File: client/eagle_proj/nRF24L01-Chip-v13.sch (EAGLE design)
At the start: 14 parts, among them IC1 7805DT, U2 ATMEGA328P-MU

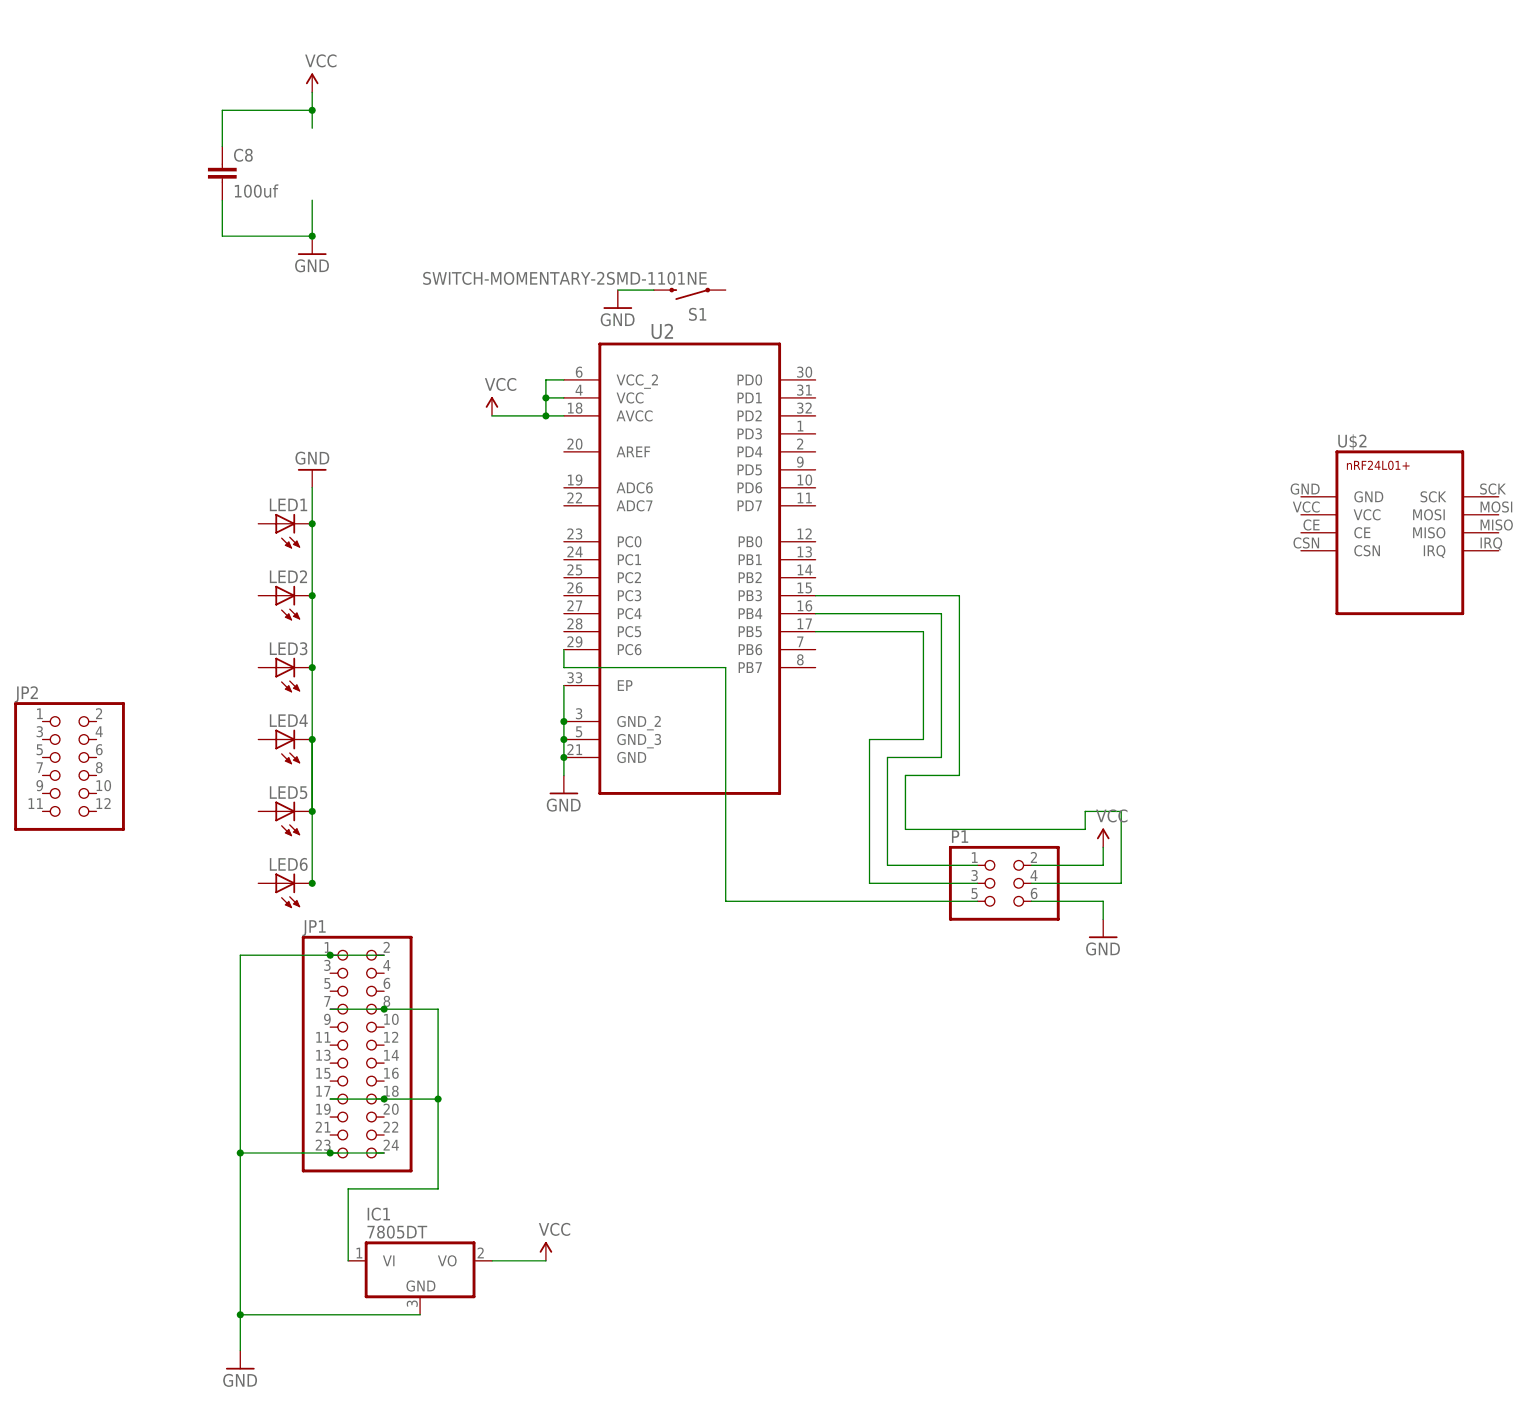
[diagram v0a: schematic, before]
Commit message: Cleanup
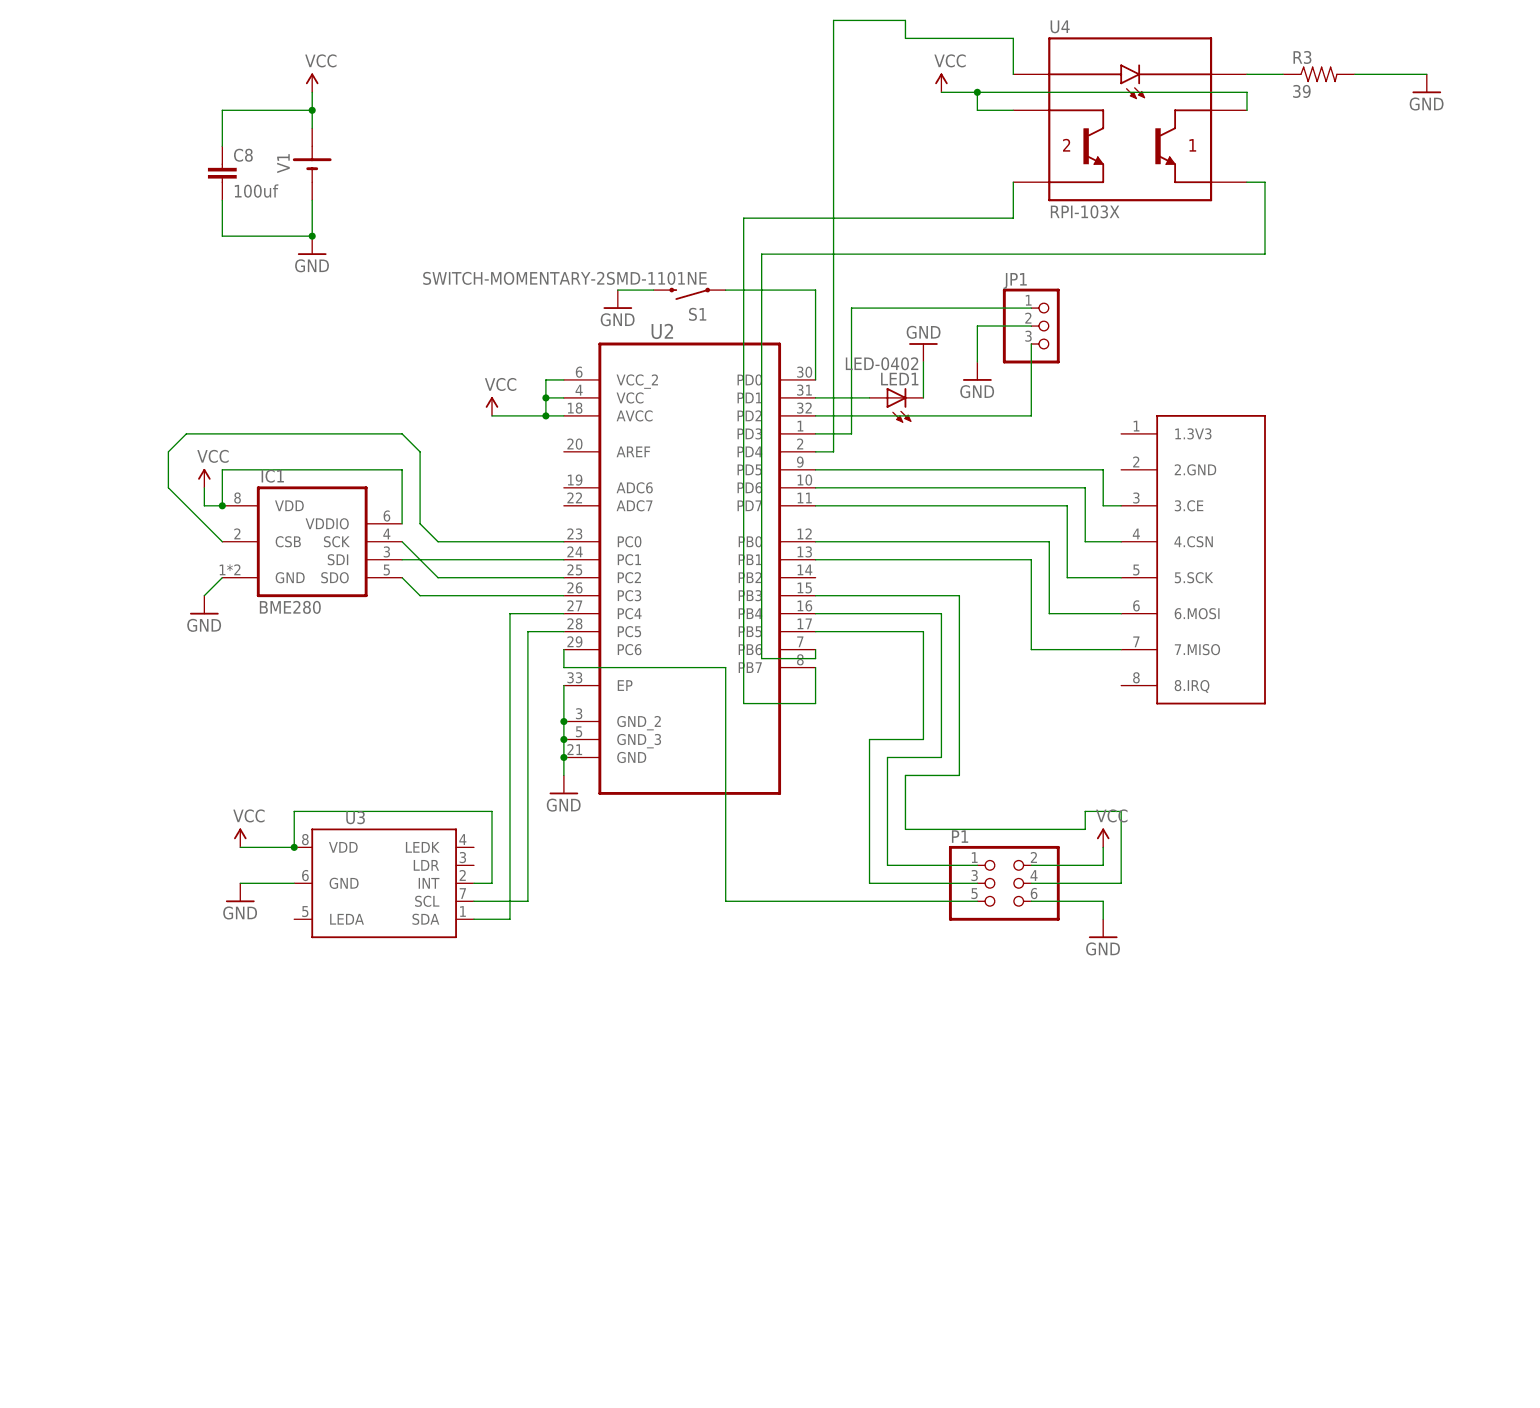
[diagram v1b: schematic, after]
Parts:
- removed JP2: (no value), pinhead:PINHD-2X6/90
- removed LED2, LED3, LED4, LED5, LED6: (no value), LilyPad-Wearables:LED1206
- removed U$2: NRF24L01+, nrf24L01:NRF24L01+
- added R3: 39, SparkFun:RESISTOR0402-RES
- added U$1: NRF24L01+, NRF:NRF24L01+
- added U3: APDS-9960, SparkFun-Sensors:APDS-9960
- added U4: RPI-103X, SparkFun-Sensors:RPI-103X
- added V1: (no value), battery_xtra:TAKACHI_BATT-CR123A
- IC1: value 7805DT -> BME280; device linear:7805DT -> bosch-bme280:BME280
- JP1: device pinhead+:PINHD-2X12SMT -> pinhead+:PINHD-1X31X03_SMT
- LED1: value (none) -> LED-0402; device LilyPad-Wearables:LED1206 -> pel_dipol_comp:LED-0402
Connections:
- new net N$15: U2.PC4, U3.SDA
- new net N$16: U2.PC5, U3.SCL
- new net N$17: IC1.SCK, U2.PC2
- new net N$18: U$1.3.CE, U2.PD5
- new net N$19: U$1.4.CSN, U2.PD6
- new net N$2: LED1.A, U2.PD1
- new net N$21: U$1.5.SCK, U2.PD7
- new net N$23: IC1.CSB, U2.PC0
- new net N$24: JP1.3, U2.PD2
- new net N$25: JP1.1, U2.PD3
- new net N$28: S1.1, U2.PD0
- new net N$29: U2.PD4, U4.ANODE
- new net N$3: IC1.SDI, U2.PC1
- new net N$30: U2.PB6, U4.E1
- new net N$31: U2.PB7, U4.E2
- new net N$32: R3.1, U4.CATHODE
- new net N$37: U$1.7.MISO, U2.PB1
- new net N$8: IC1.SDO, U2.PC3
- net GND: now also R3.2, U3.GND, V1.-; no longer JP1.1, JP1.23, JP1.24, LED2.C, LED3.C, LED4.C, LED5.C, LED6.C
- net N$1: now also U$1.6.MOSI, U2.PB0; no longer IC1.VI, JP1.17, JP1.18, JP1.7, JP1.8
- net VCC: now also IC1.VDD, IC1.VDDIO, U3.INT, U3.VDD, U4.C1, U4.C2, V1.+; no longer IC1.VO
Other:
- moved on the sheet: LED1
